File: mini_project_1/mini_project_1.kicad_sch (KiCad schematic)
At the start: 15 parts, among them J1 480370001, U2 MCP1700x-330xxTT, U3 MCP602

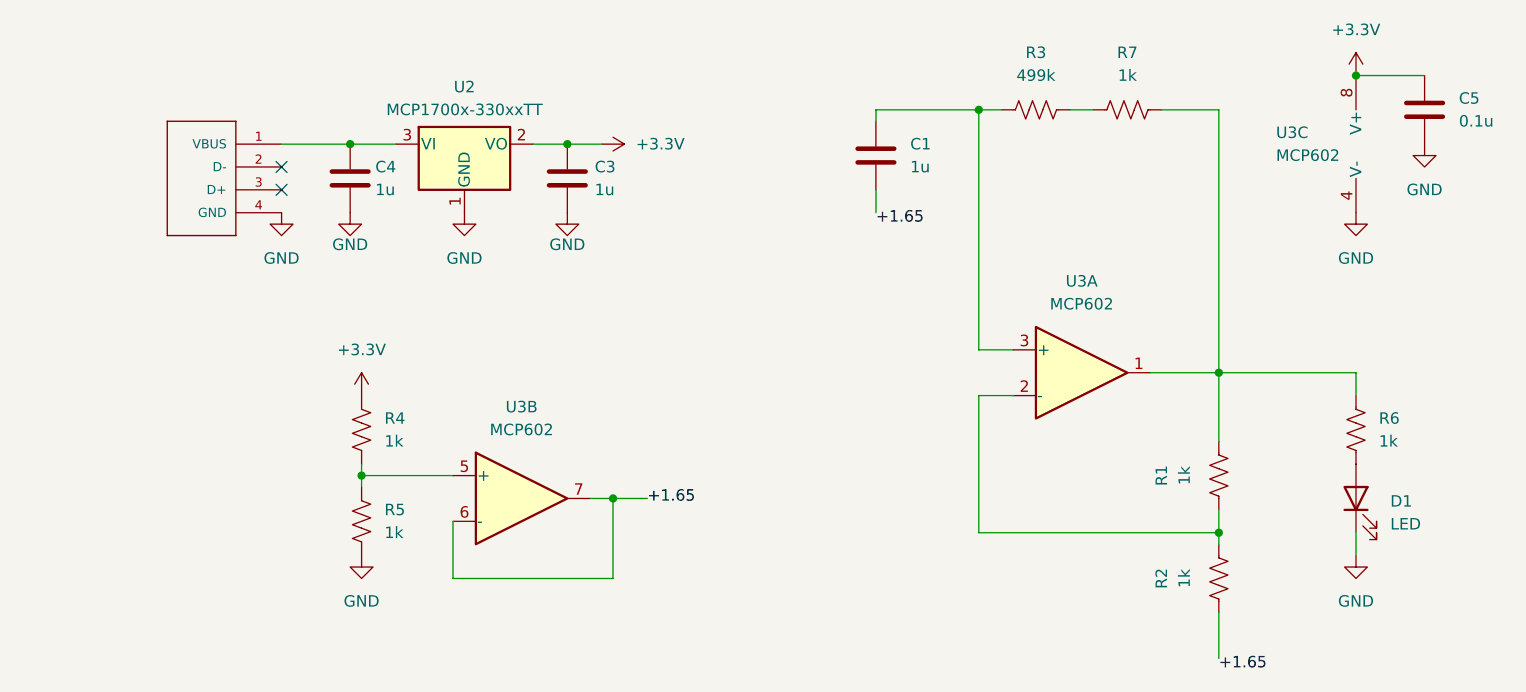
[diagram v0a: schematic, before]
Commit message: Modify schematic, layout, and add report
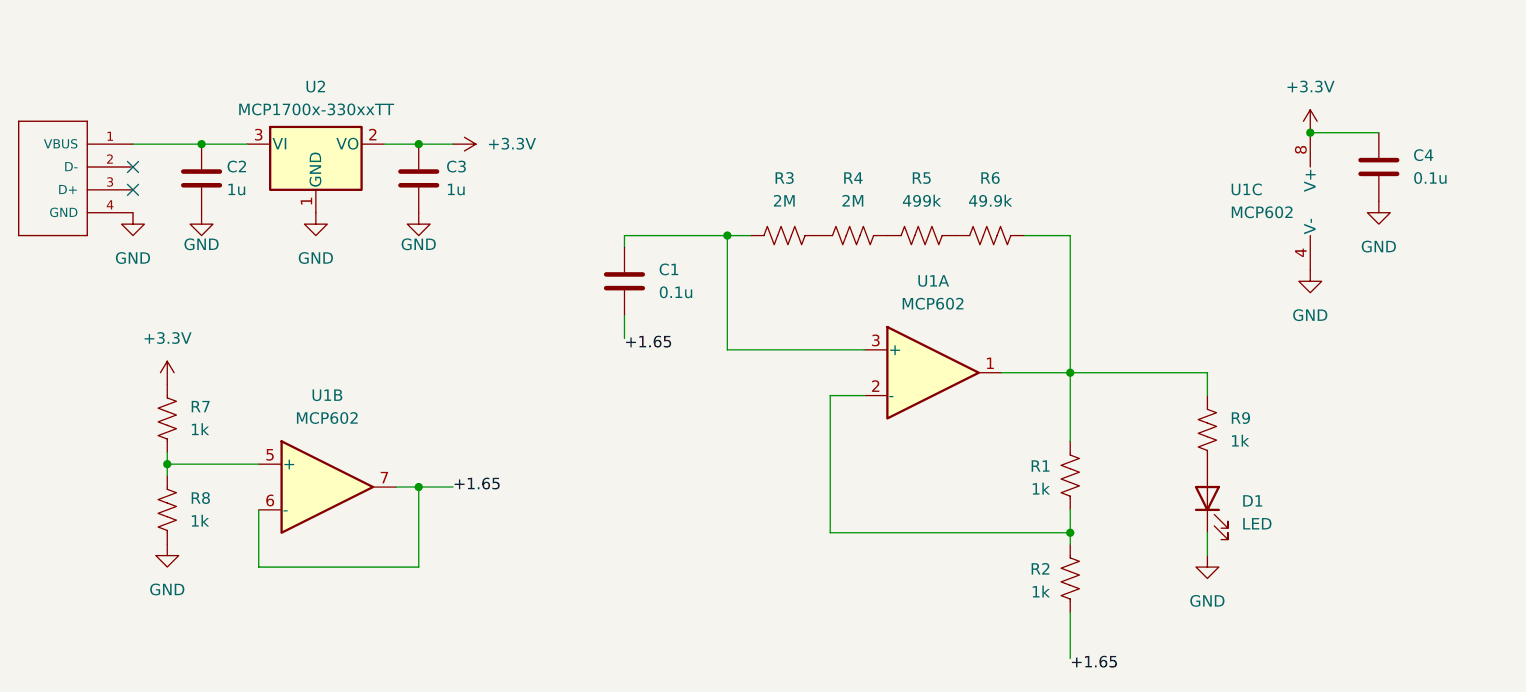
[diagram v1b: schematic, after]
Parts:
- added R5: 499k, Resistor_SMD:R_0603_1608Metric, symbol Device:R_US
- added R6: 49.9k, Resistor_SMD:R_0603_1608Metric, symbol Device:R_US
- C1: value 1u -> 0.1u
- R1, R2: footprint Diode_SMD:D_0603_1608Metric -> Resistor_SMD:R_0603_1608Metric
- R3: value 499k -> 2M; footprint Diode_SMD:D_0603_1608Metric -> Resistor_SMD:R_0603_1608Metric
- R4: renamed from R7; value 1k -> 2M; footprint Diode_SMD:D_0603_1608Metric -> Resistor_SMD:R_0603_1608Metric
- R7: renamed from R4; footprint Diode_SMD:D_0603_1608Metric -> Resistor_SMD:R_0603_1608Metric
- R8: renamed from R5; footprint Diode_SMD:D_0603_1608Metric -> Resistor_SMD:R_0603_1608Metric
- R9: renamed from R6; footprint Diode_SMD:D_0603_1608Metric -> Resistor_SMD:R_0603_1608Metric
- renumbered C4 to C2, C5 to C4, U3 to U1
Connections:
- net at R1.2, R9.1, U1.1: now also R6.2; no longer R4.2
- new net: R4.2, R5.1
- new net: R5.2, R6.1
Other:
- moved on the sheet: C1, C2, C3, C4, D1, R1, R2, R3, R4, R7, R8, R9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
